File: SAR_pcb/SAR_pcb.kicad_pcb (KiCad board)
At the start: 4 copper layers, 87.6 x 63.5 mm, 38 parts, among them J1 Conn_Coaxial_Power, J10 Conn_Coaxial, J2 Conn_Coaxial_Power, J3 Conn_02x10_Top_Bottom, J6 Conn_01x02_Male, J7 Conn_01x02_Male, J8 Conn_01x02_Male, J9 Conn_Coaxial, SW1 SW_Push, U2 10B_SAR

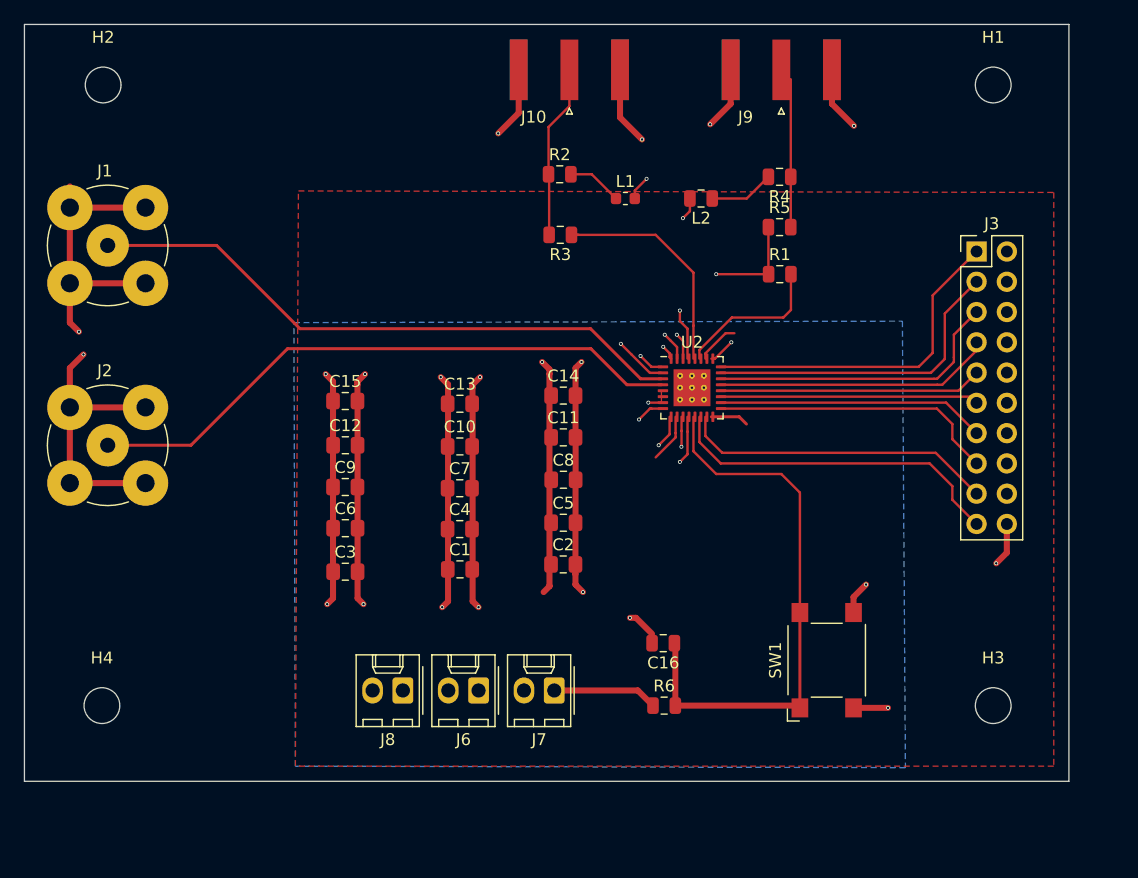
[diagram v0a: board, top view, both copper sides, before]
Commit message: Draft 2 of Layout
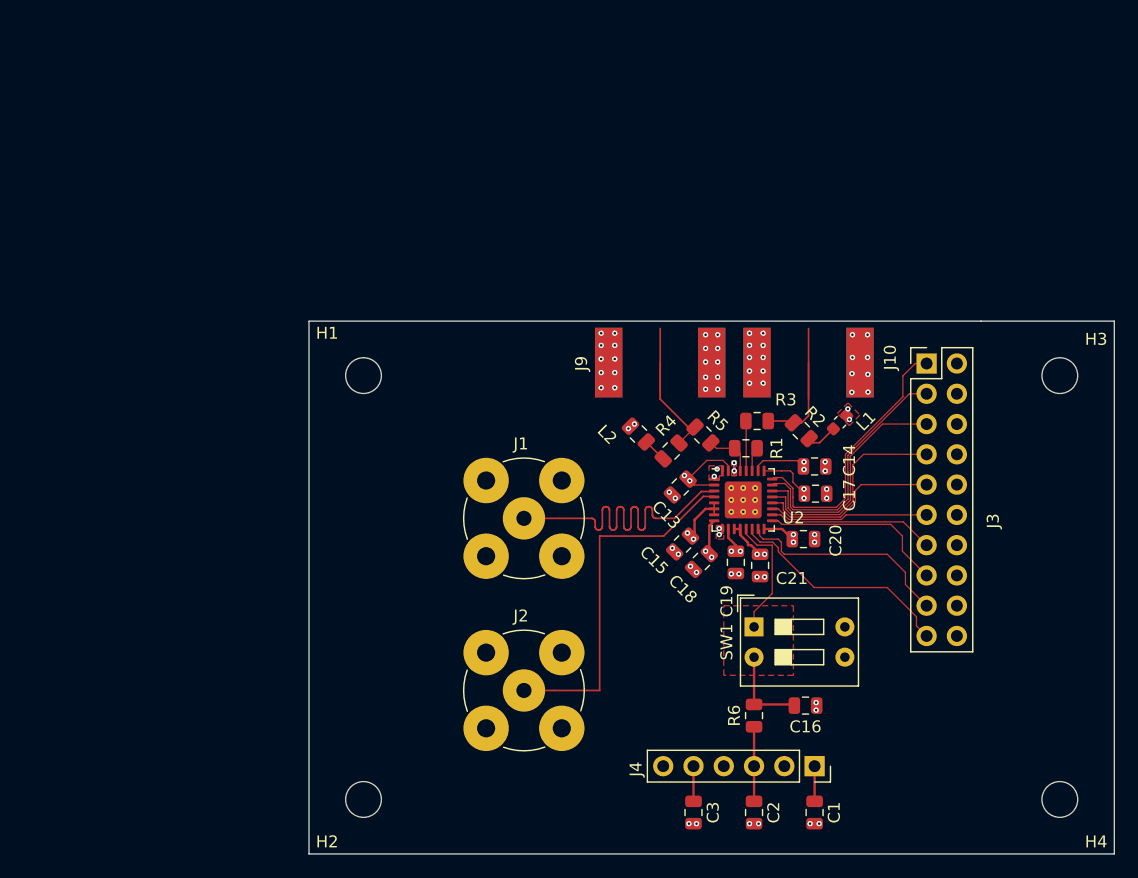
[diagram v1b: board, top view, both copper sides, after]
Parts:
- removed C10, C11, C12: 0.01, Capacitor_SMD:C_0805_2012Metric_Pad1.15x1.40mm_HandSolder
- removed C4, C5, C6: 1u, Capacitor_SMD:C_0805_2012Metric_Pad1.15x1.40mm_HandSolder
- removed C7, C8, C9: 0.1u, Capacitor_SMD:C_0805_2012Metric_Pad1.15x1.40mm_HandSolder
- removed J6, J7, J8: Conn_01x02_Male, Connector_Molex:Molex_KK-254_AE-6410-02A_1x02_P2.54mm_Vertical
- added C17: 0.01u, Capacitor_SMD:C_0805_2012Metric, F.Cu at (155.3, 92.7)
- added C18: 0.01u, Capacitor_SMD:C_0805_2012Metric, F.Cu at (145.7, 98.4)
- added C19: 0.01u, Capacitor_SMD:C_0805_2012Metric, F.Cu at (148.6, 98.5)
- added C20: 0.01u, Capacitor_SMD:C_0805_2012Metric, F.Cu at (154.3, 96.5)
- added C21: 0.01u, Capacitor_SMD:C_0805_2012Metric, F.Cu at (150.6, 98.7)
- added J4: Conn_01x06, Connector_PinSocket_2.54mm:PinSocket_1x06_P2.54mm_Vertical, F.Cu at (155.2, 115.6)
- C1, C2, C3: footprint Capacitor_SMD:C_0805_2012Metric_Pad1.15x1.40mm_HandSolder -> Capacitor_SMD:C_0805_2012Metric
- C13, C14, C15: value 0.001u -> 0.01u; footprint Capacitor_SMD:C_0805_2012Metric_Pad1.15x1.40mm_HandSolder -> Capacitor_SMD:C_0805_2012Metric
- J10, J9: footprint Connector_Coaxial:SMA_Amphenol_132289_EdgeMount -> SAR_pcb:CustomSMA
- SW1: footprint Button_Switch_SMD:SW_SPST_Omron_B3FS-100xP -> Button_Switch_THT:SW_DIP_SPSTx02_Slide_9.78x7.26mm_W7.62mm_P2.54mm
- moved H4 80.8 mm to (175.8, 118.4)
- moved H2 63.8 mm to (117.3, 118.4)
- moved H1 58.2 mm to (117.3, 82.8)
- moved J1 41.8 mm to (130.8, 94.8)
- moved J2 40.5 mm to (130.8, 109.2)
- moved C1 36.1 mm to (155.2, 119.5), turned to 270 degrees
- moved C3 35.5 mm to (145.0, 119.5), turned to 270 degrees
- moved J10 31.7 mm to (154.7, 81.7), turned to 0 degrees
- moved C15 30.7 mm to (144.1, 96.9), turned to 225 degrees
- moved R2 29.6 mm to (154.1, 87.4), turned to 315 degrees
- moved H3 28.2 mm to (175.8, 82.8)
- moved J9 26.6 mm to (142.2, 81.7), turned to 0 degrees
- moved C2 26.3 mm to (150.1, 119.5), turned to 270 degrees
- moved L1 26.0 mm to (157.3, 86.7), turned to 45 degrees
- moved R4 24.7 mm to (143.2, 89.1), turned to 225 degrees
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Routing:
- net GND: track 159.3 -> 0.16 mm, vias 22 -> 72
- net RST: track 47.1 -> 17.9 mm
- net VDDPST: track 39.4 -> 15.7 mm, vias 1 -> 6
- net VIN-: track 51.1 -> 30.3 mm
- net VIN+: track 51.1 -> 30.3 mm
- net VDD: track 37.7 -> 21.0 mm
- net CLK_S_FILT: track 19.4 -> 4.19 mm
- net VREF: track 21.9 -> 7.48 mm, vias 3 -> 2
- net CLK_FILT: track 17.0 -> 4.28 mm, vias 2 -> 0
- net Net-(R1-Pad2): track 12.8 -> 2.07 mm
- net D9: track 28.9 -> 19.2 mm
- net D8: track 26.8 -> 18.1 mm
- net D7: track 24.2 -> 15.6 mm
- net D6: track 22.6 -> 14.0 mm
- net D5: track 21.8 -> 13.5 mm
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- added copper zone on F.Cu, net GND
- added copper zone on F.Cu, net RST
- added copper zone on VDD, net VDDPST
- added copper zone on VDD, net VREF
- removed copper zone on F.Cu, net VDDPST
- removed copper zone on B.Cu, net VREF
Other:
- board size 87.6 x 63.5 mm -> 67.6 x 44.7 mm
- net class Default: via_dia 0.3302 -> 0.4572
- rule via_min_size: 0.3302 -> 0.4572
